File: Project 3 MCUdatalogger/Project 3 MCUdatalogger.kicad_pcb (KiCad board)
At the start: 2 copper layers, 53.1 x 35.7 mm, 30 parts, among them J1 Conn_01x04_Pin, J2 Conn_01x09_Pin, J3 Conn_01x04_Pin, J4 Conn_02x03_Odd_Even, U1 24LC1025, U2 DS1337S_, U3 24LC1025, U4 ATMEGA328P-AU, Y1 32.768 KHz, Y2 16 MHz

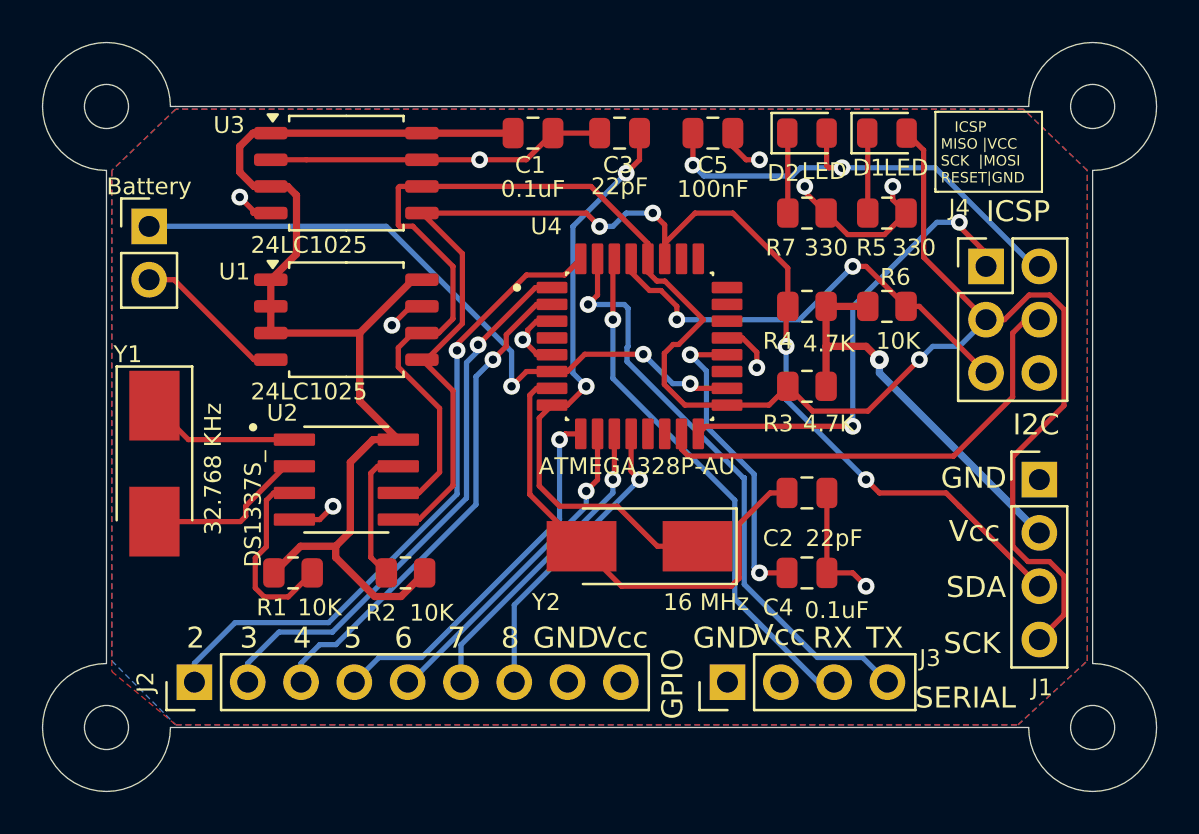
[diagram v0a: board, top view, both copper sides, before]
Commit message: Routing
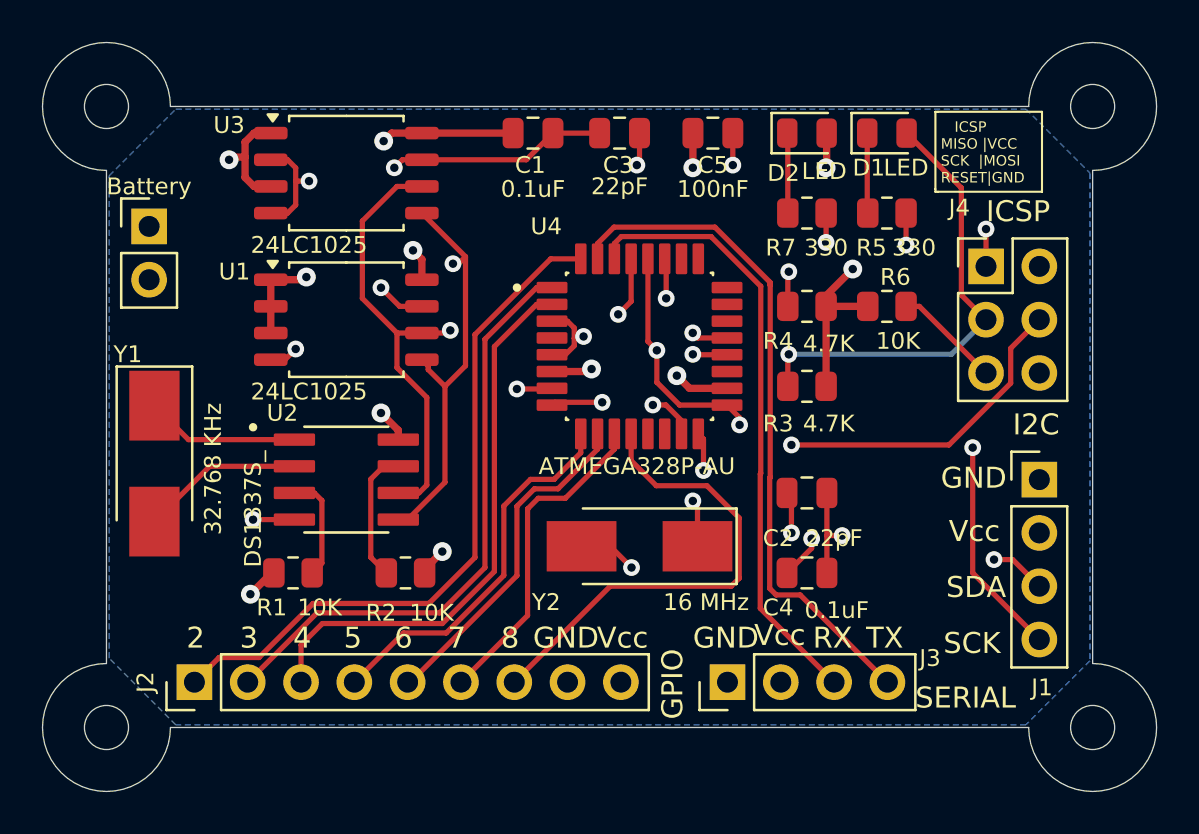
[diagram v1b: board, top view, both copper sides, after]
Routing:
- net /Vcc: track 131.4 -> 38.0 mm, vias 6 -> 12
- net GND: track 52.4 -> 35.7 mm, vias 10 -> 11
- net /D8: track 14.5 -> 23.2 mm, vias 1 -> 0
- net /SCK: track 94.2 -> 86.5 mm, vias 1 -> 5
- net /MISO: track 22.6 -> 27.8 mm
- net /RESET: track 22.0 -> 26.7 mm, vias 2 -> 1
- net /RX: track 25.0 -> 29.2 mm, vias 1 -> 0
- net Net-(U2-~{INTA}): track 9.24 -> 5.10 mm
- net Net-(U4-AREF): track 14.8 -> 18.8 mm
- net /TX: track 28.7 -> 32.4 mm, vias 1 -> 0
- net /D4: track 23.8 -> 26.7 mm, vias 1 -> 0
- net /MOSI: track 22.4 -> 25.0 mm, vias 0 -> 2
- net Net-(U4-PB6): track 23.4 -> 25.6 mm, vias 0 -> 3
- net Net-(U4-PB7): track 28.5 -> 26.3 mm, vias 2 -> 3
- net /D3: track 26.8 -> 28.7 mm, vias 1 -> 0
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- added copper zone on In2.Cu, net /Vcc
- removed copper zone on F.Cu, net /Vcc
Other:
- copper layers 2 -> 4
